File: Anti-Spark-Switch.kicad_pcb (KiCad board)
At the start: 2 copper layers, 63.2 x 42 mm, 16 parts, among them P1 Pad_Conn, P2 Pad_Conn, P3 Screw_Terminal, P4 Screw_Terminal, P5 Pad_Conn, P6 Pad_Conn, P7 CONN_01X02, Q1 IRFS7530, Q2 IRFS7530, Q3 IRFS7530, SW1 SW_PUSH

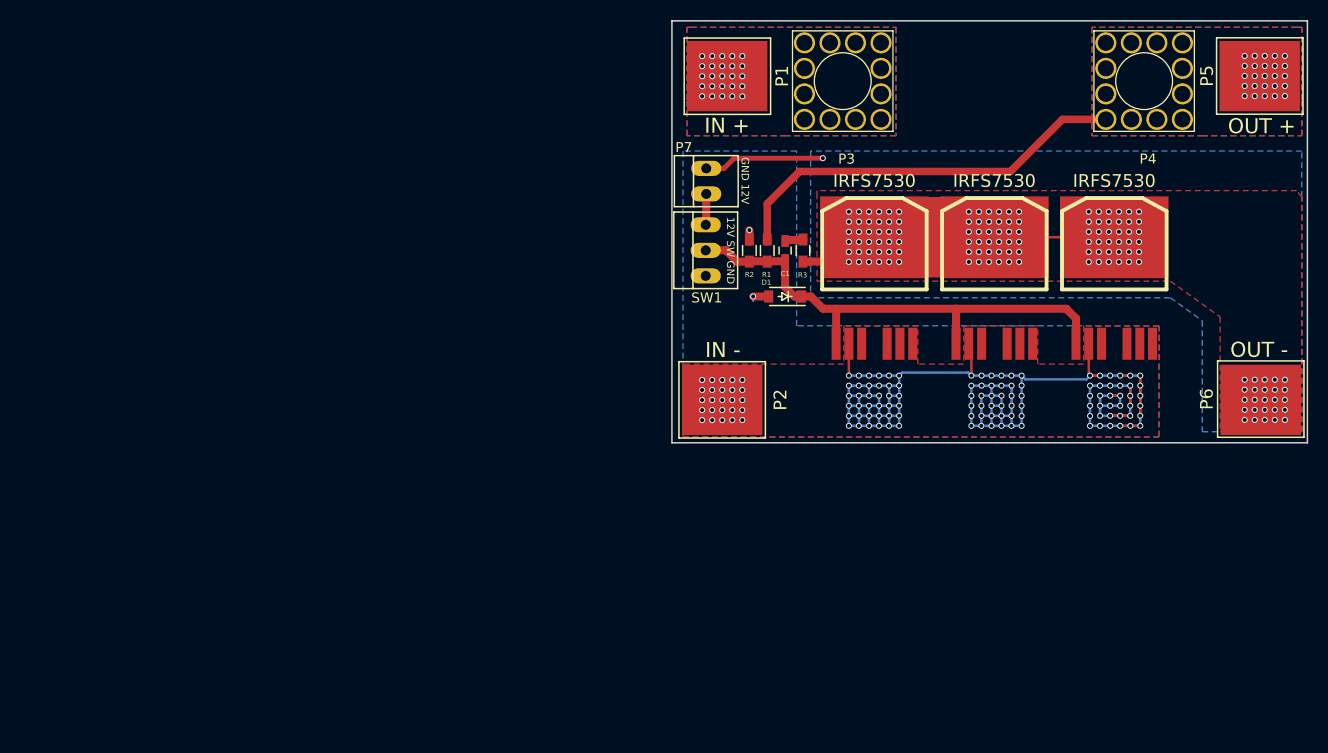
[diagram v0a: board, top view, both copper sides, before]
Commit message: updated the PCB per new schematic changes and general improvements
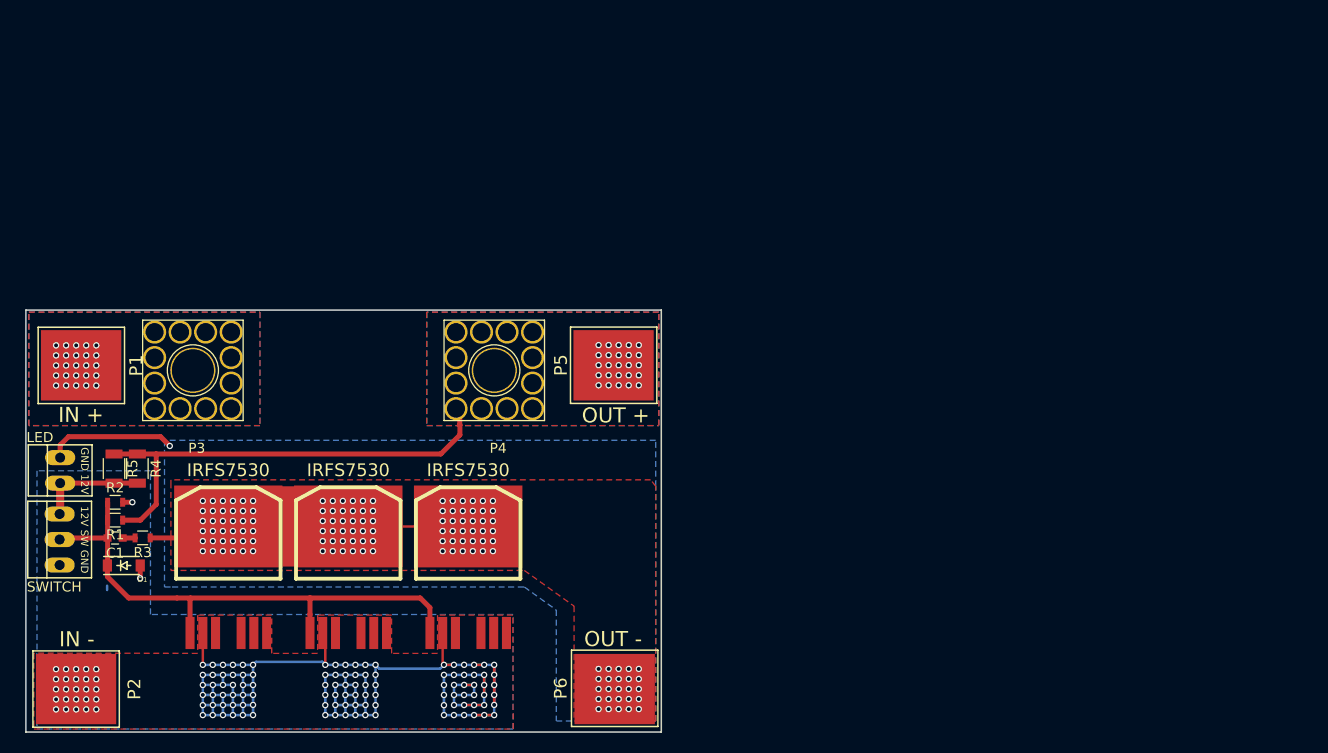
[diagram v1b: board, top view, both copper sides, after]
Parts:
- added R4: 16.5K, Resistors_SMD:R_1206, F.Cu at (126.8, 92.6)
- added R5: 16.5K, Resistors_SMD:R_1206, F.Cu at (124.5, 92.6)
- C1: footprint Capacitors_SMD:C_0603_HandSoldering -> Capacitors_SMD:C_0603
- P3, P4: footprint Spark_Parts:M5_Screw_Terminal_12_pin -> sparkparts:M5_Screw_Terminal_12_pin
- R1, R2, R3: footprint Resistors_SMD:R_0603_HandSoldering -> Resistors_SMD:R_0603
- moved C1 72.6 mm to (124.6, 99.5), turned to 180 degrees
- moved R3 71.7 mm to (127.3, 99.5), turned to 180 degrees
- moved D1 71.1 mm to (125.4, 102.2), turned to 0 degrees
- moved P3 70.8 mm to (132.3, 82.8)
- moved P4 70.8 mm to (162.3, 82.8)
- moved LED 70.5 mm to (119.1, 92.7)
- moved P1 70.5 mm to (121.2, 82.3)
- moved P2 70.5 mm to (120.7, 114.5)
- moved P5 70.5 mm to (174.2, 82.3)
- moved P6 70.5 mm to (174.3, 114.4)
- moved Q2 70.5 mm to (147.8, 104.2)
- moved Q3 70.5 mm to (159.7, 104.2)
- moved SWITCH 70.5 mm to (119.1, 99.6)
- moved Q1 70.5 mm to (135.8, 104.2)
- moved R1 70.2 mm to (124.6, 97.7), turned to 180 degrees
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- renumbered P7 to LED, SW1 to SWITCH
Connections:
- net +12V renamed Net-(P7-Pad1)
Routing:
- net Net-(P7-Pad1): track 3.09 -> 10.8 mm
- net Net-(P4-Pad1): track 67.8 -> 73.7 mm
- net Net-(C1-Pad2): track 51.0 -> 55.1 mm
- net Net-(P6-Pad1): track 116.5 -> 120.5 mm
- net Net-(C1-Pad1): track 1.78 -> 1.25 mm
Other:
- net class Default: clearance 0.2 -> 0
- rule trace_clearance: 0.2 -> 0
- board text added: "AntiSpark"
- board text added: "Ver: 1.3 Date: 4/21/18"
- board text removed: "GiS AntiSpark"
- board text removed: "Ver: 1.2 Date: 2/17"
